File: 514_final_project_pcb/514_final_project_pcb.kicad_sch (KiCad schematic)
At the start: 31 parts, among them Q1 BC847, U1 XIAO-ESP32-C3-DIP, U2 XIAO-ESP32-C3-DIP

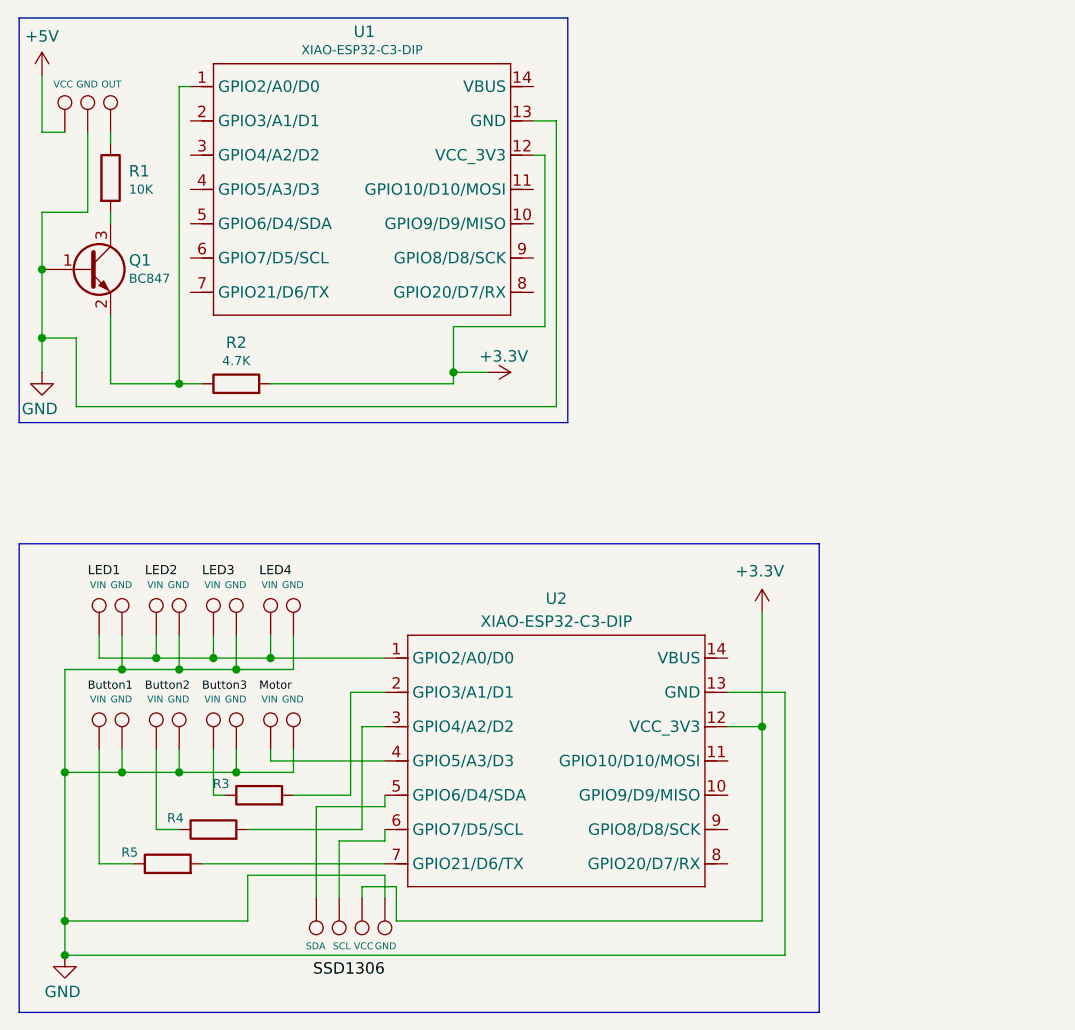
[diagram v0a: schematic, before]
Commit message: updated files
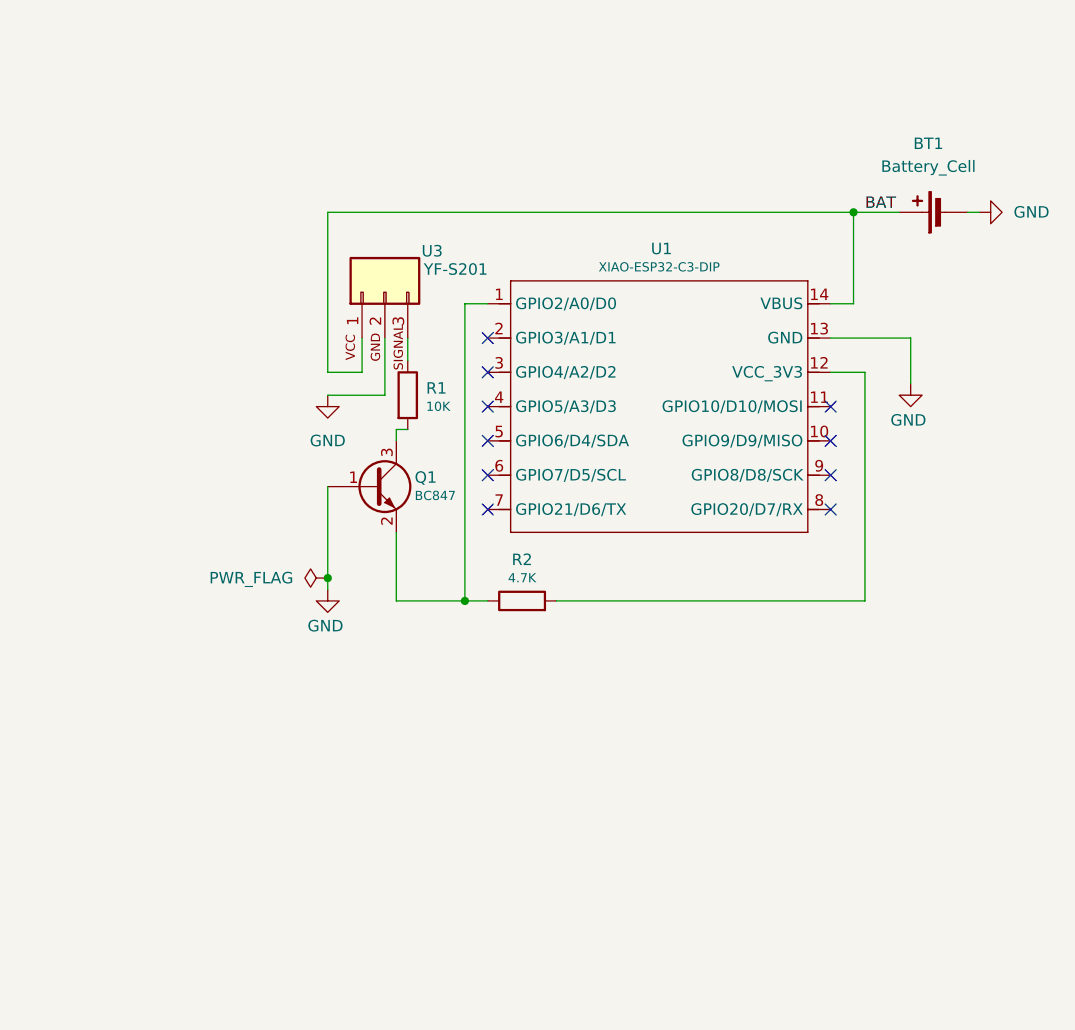
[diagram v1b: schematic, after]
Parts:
- removed R3, R4, R5: 10K, Resistor_SMD:R_0603_1608Metric, symbol Device:R
- removed TP1, TP10: VCC, symbol Connector:TestPoint
- removed TP11, TP15, TP17, TP19, TP2, TP21, TP23, TP5, TP7, TP9: GND, symbol Connector:TestPoint
- removed TP12: SCL, symbol Connector:TestPoint
- removed TP13: SDA, symbol Connector:TestPoint
- removed TP14, TP16, TP18, TP20, TP22, TP4, TP6, TP8: VIN, symbol Connector:TestPoint
- removed TP3: OUT, symbol Connector:TestPoint
- removed U2: XIAO-ESP32-C3-DIP, Module:MOUDLE14P-XIAO-DIP-SMD, symbol Seeed_Studio_XIAO_Series:XIAO-ESP32-C3-DIP
- added BT1: Battery_Cell, Connector_JST:JST_NV_B02P-NV_1x02_P5.00mm_Vertical, symbol Device:Battery_Cell
- added U3: YF-S201, Connector_PinSocket_2.54mm:PinSocket_1x03_P2.54mm_Vertical, symbol Connector_Generic:Conn_01x03
- U1: footprint Module:MOUDLE14P-XIAO-DIP-SMD -> Seeed Studio XIAO Series Library:XIAO-ESP32C3-DIP
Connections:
- net GND: now also BT1.2 (-), U3.2 (GND)
- net at R1.1: now also U3.3 (SIGNAL)
- net BAT: now reaches U1.14 (VBUS)
- net BAT: now also BT1.1 (+), U3.1 (VCC)
- net +3.3V: no longer names the net of R2.2, U1.12 (VCC_3V3)
- no-connect marks 0 -> 10
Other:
- company: (none) -> Marjorie Yang
- title: (none) -> 514 Sensing Device Schematic
- moved on the sheet: Q1, R1, R2, U1
